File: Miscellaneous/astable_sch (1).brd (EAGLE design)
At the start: 160 x 100 mm, 6 parts, among them IC1 LM555N

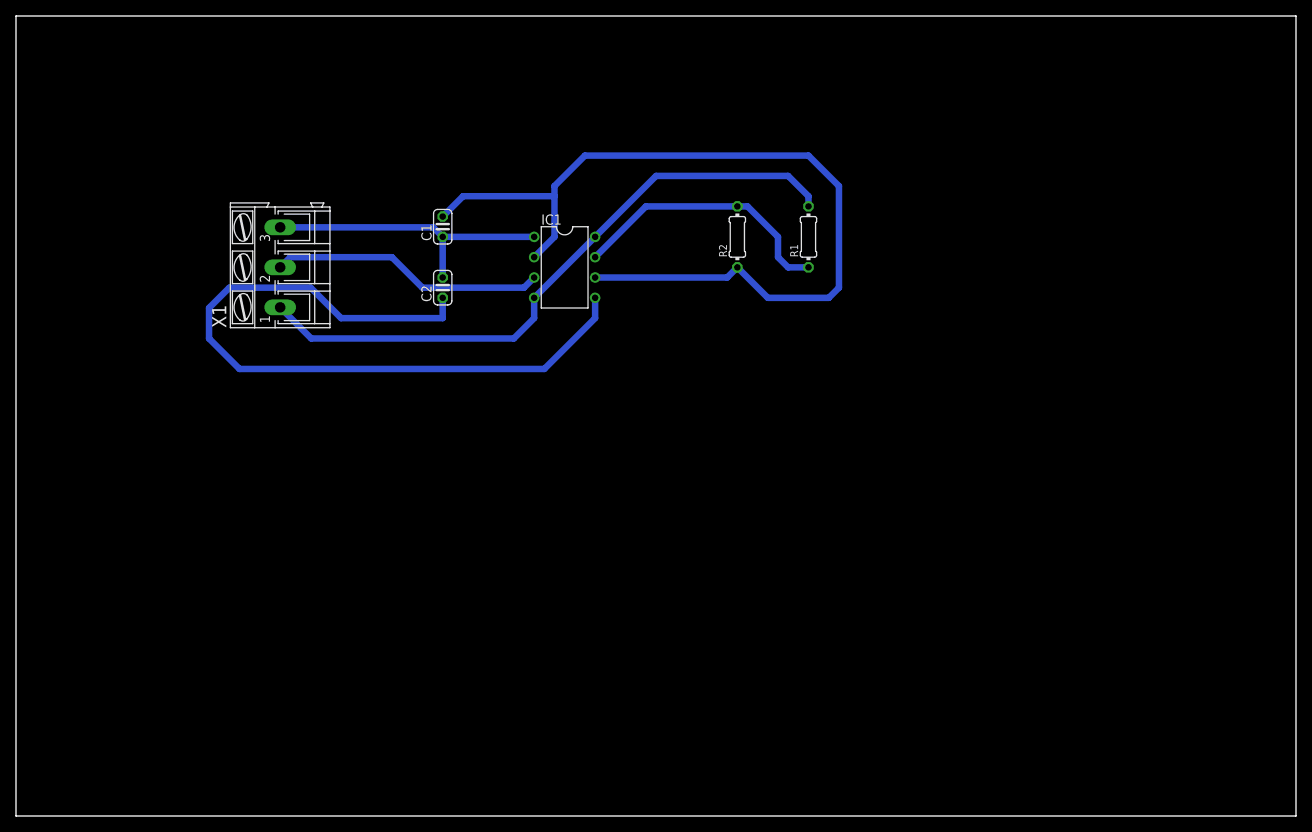
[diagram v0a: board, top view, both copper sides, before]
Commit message: Fixed the PCB design
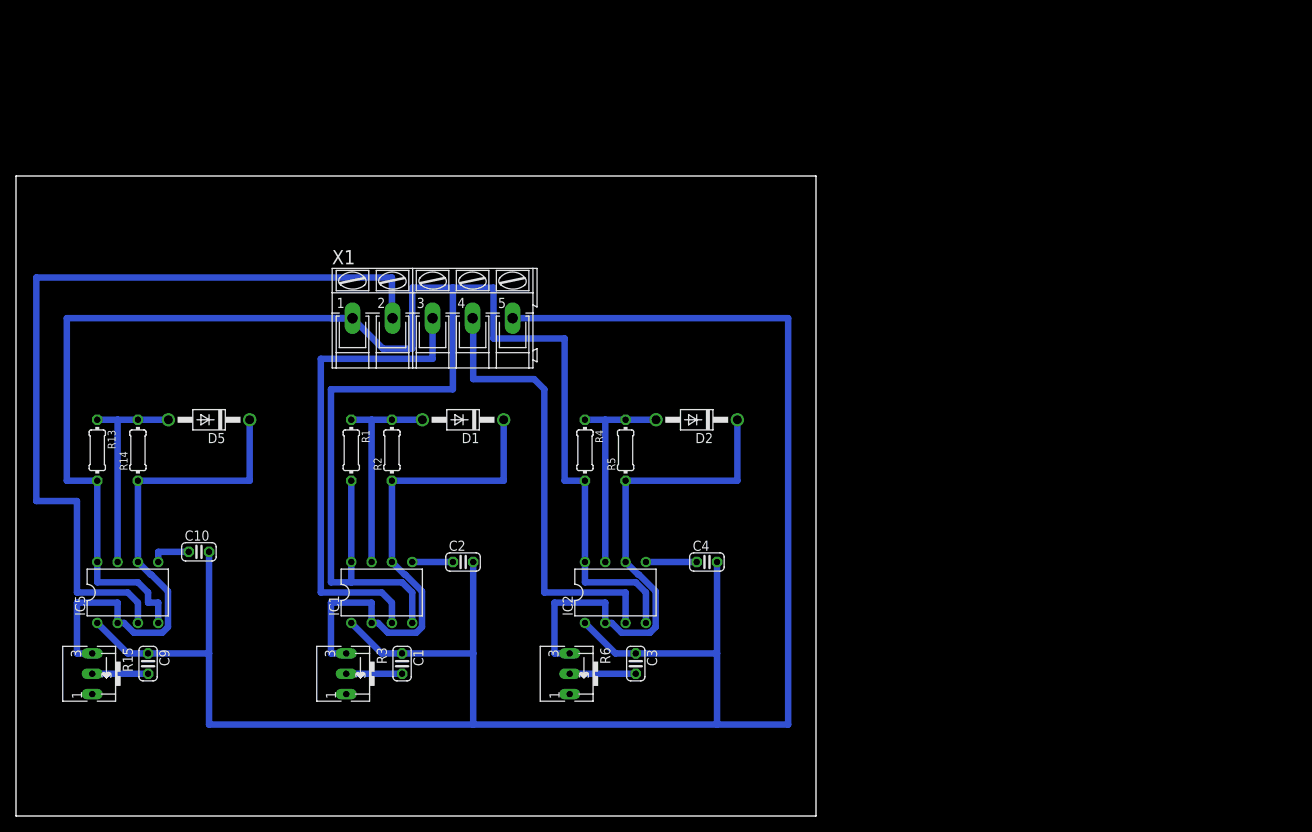
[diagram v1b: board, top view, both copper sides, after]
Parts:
- added C10, C3, C4, C9: (no value), rcl:C025-024X044
- added D1, D2, D5: 1N4004, diode:DO41-10
- added IC2, IC5: LM555N, linear:DIL08
- added R13, R14, R4, R5: (no value), rcl:0204/7
- added R15, R3, R6: (no value), pot:B25V
- X1: device con-ptr500:AK300/3 -> con-ptr500:AK300/5
- moved R1 63.1 mm to (41.9, 45.7), turned to 270 degrees
- moved C1 54.8 mm to (48.3, 19.1), turned to 270 degrees
- moved R2 50.8 mm to (47.0, 45.7)
- moved IC1 46.6 mm to (45.7, 27.9), turned to 0 degrees
- moved C2 34.4 mm to (55.9, 31.8), turned to 0 degrees
- moved X1 20.1 mm to (52.1, 62.2), turned to 0 degrees
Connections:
- new net N$1: D1.A, IC1.7, R1.1, R2.2
- new net N$10: C3.2, R6.S
- new net N$21: D5.A, IC5.7, R13.1, R14.2
- new net N$22: D5.C, IC5.2, IC5.6, R14.1, R15.E
- new net N$23: C10.1, IC5.5
- new net N$24: IC5.3, X1.2
- new net N$25: C9.2, R15.S
- new net N$5: C1.2, R3.S
- new net N$6: D2.A, IC2.7, R4.1, R5.2
- new net N$7: D2.C, IC2.2, IC2.6, R5.1, R6.E
- new net N$8: C4.1, IC2.5
- net GND: now also C10.2, C3.1, C4.2, C9.1, IC2.1, IC5.1, X1.5; no longer X1.3
- net N$2: now also D1.C, IC1.2, IC1.6, R2.1, R3.E; no longer IC1.7, R1.1, R2.2
- net N$4: now also IC1.3, X1.3; no longer C1.2, IC1.2, IC1.6, R2.1
- net N$9: now also IC2.3, X1.4; no longer IC1.3, X1.2
- net VCC: now also IC2.4, IC2.8, IC5.4, IC5.8, R13.2, R4.2
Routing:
- net GND: track 37.3 -> 270.3 mm
- net VCC: track 79.9 -> 253.5 mm
- net N$24: track 0.00 -> 104.7 mm
- net N$3: track 93.2 -> 5.08 mm
- net N$7: track 0.00 -> 65.7 mm
- net N$22: track 0.00 -> 64.5 mm
- net N$4: track 109.5 -> 60.2 mm
- net N$2: track 33.9 -> 64.5 mm
- net N$6: track 0.00 -> 26.7 mm
- net N$21: track 0.00 -> 26.7 mm
- net N$1: track 0.00 -> 26.7 mm
- net N$9: track 34.4 -> 56.4 mm
- net N$10: track 0.00 -> 8.25 mm
- net N$25: track 0.00 -> 6.99 mm
- net N$5: track 0.00 -> 6.98 mm
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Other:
- board size 160 x 100 mm -> 100 x 80 mm
